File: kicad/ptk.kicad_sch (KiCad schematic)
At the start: 25 parts, among them J0 nice!view, U0 ProMicro-kbd

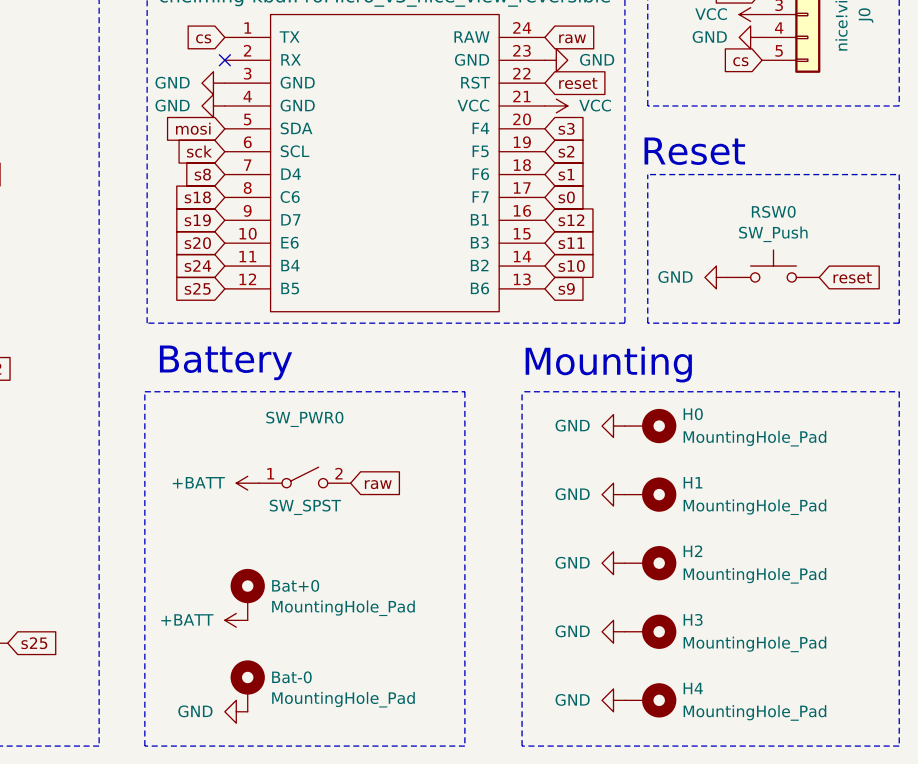
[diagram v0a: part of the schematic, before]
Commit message: add'l routing
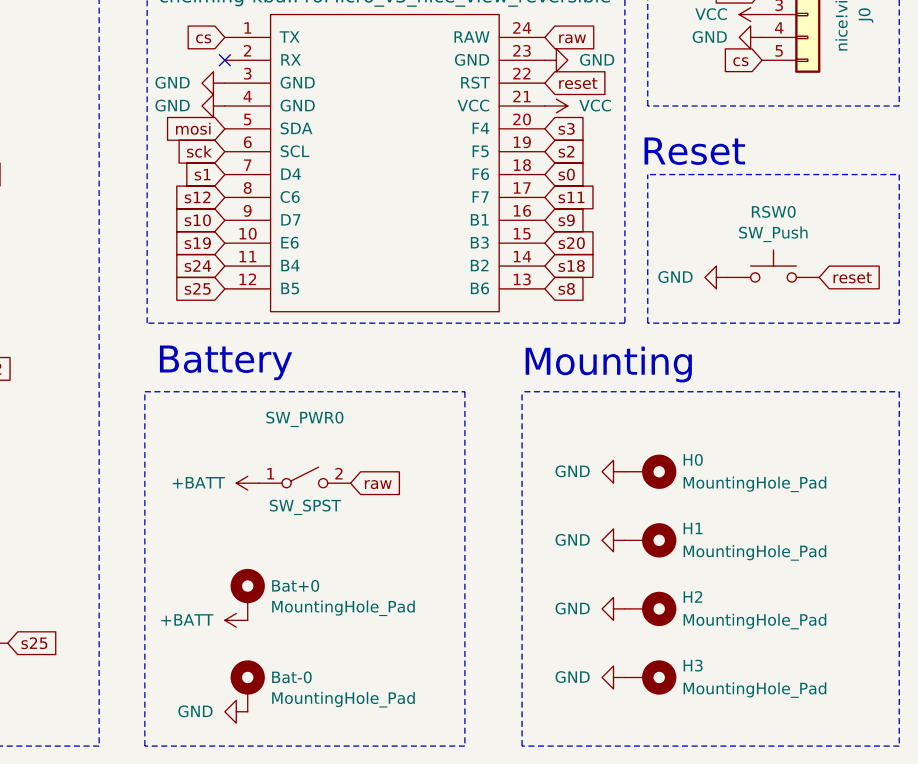
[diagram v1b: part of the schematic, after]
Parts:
- removed H4: MountingHole_Pad, MountingHole:MountingHole_2.2mm_M2_Pad_Via, symbol Mechanical:MountingHole_Pad
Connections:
- net s0: now also U0.18 (F6); no longer U0.17 (F7)
- net s1: now also U0.7 (D4); no longer U0.18 (F6)
- net s10: now also U0.9 (D7); no longer U0.14 (B2)
- net s11: now also U0.17 (F7); no longer U0.15 (B3)
- net s12: now also U0.8 (C6); no longer U0.16 (B1)
- net s18: now also U0.14 (B2); no longer U0.8 (C6)
- net s19: now also U0.10 (E6); no longer U0.9 (D7)
- net s20: now also U0.15 (B3); no longer U0.10 (E6)
- net s8: now also U0.13 (B6); no longer U0.7 (D4)
- net s9: now also U0.16 (B1); no longer U0.13 (B6)
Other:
- moved on the sheet: H0, H1, H2, H3

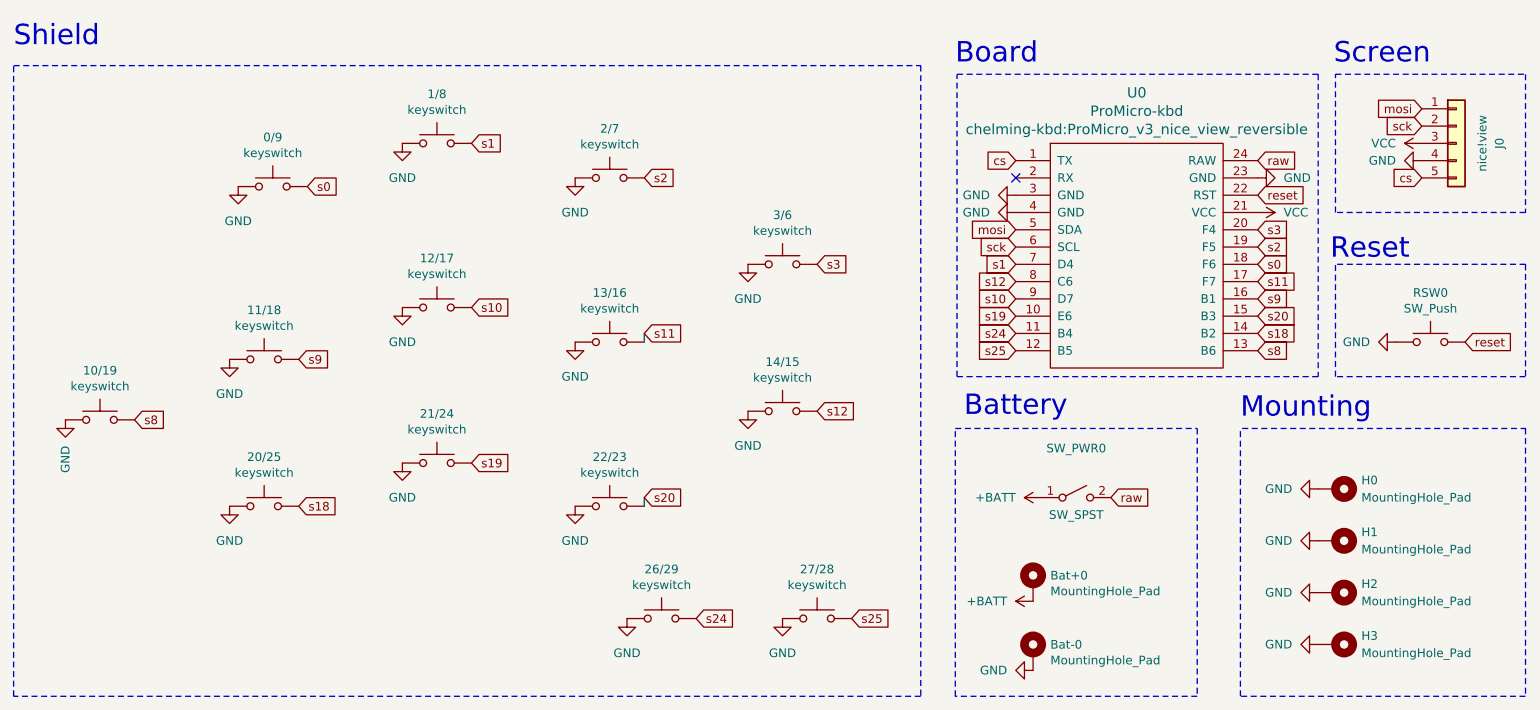
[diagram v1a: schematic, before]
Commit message: added boxes around the keys on the schematic because I'm weird like that
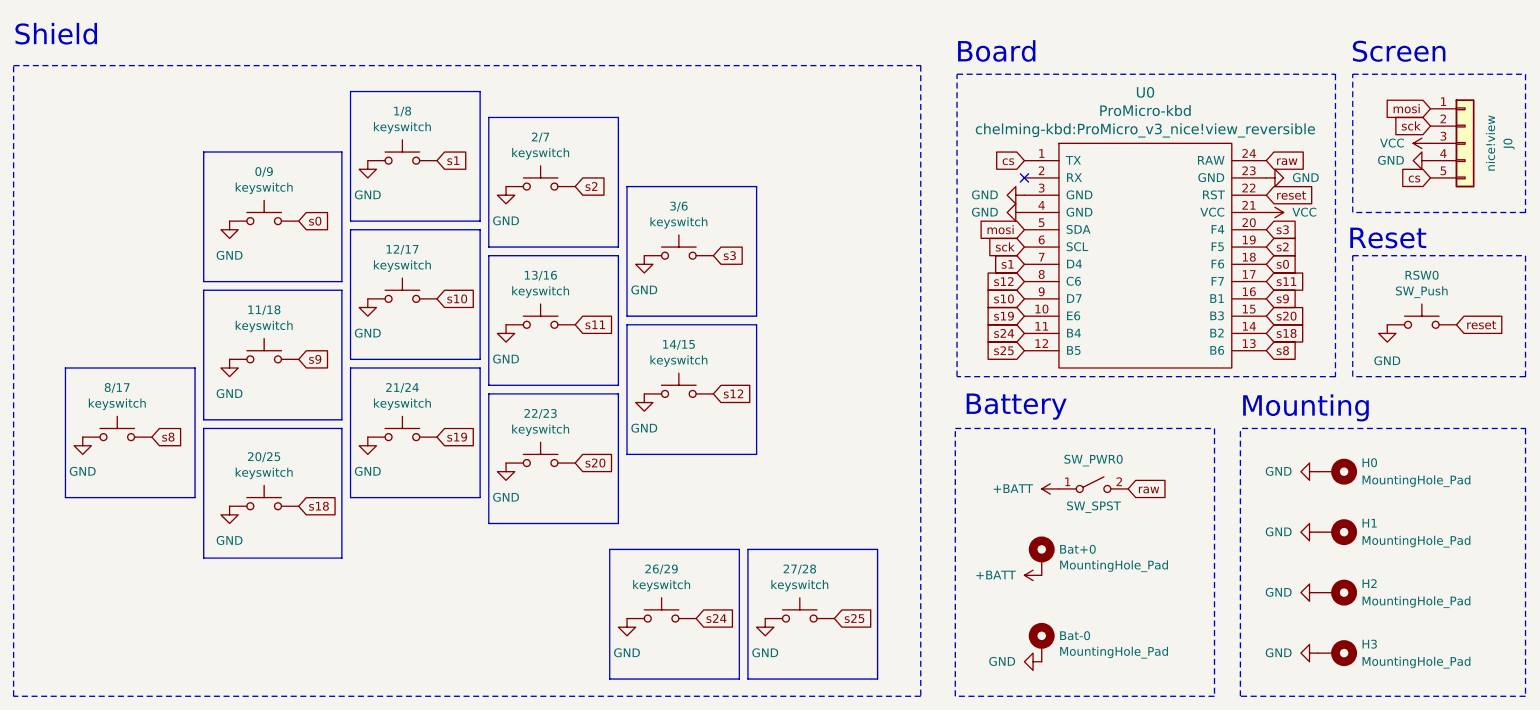
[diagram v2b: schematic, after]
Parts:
- removed 10/19: keyswitch, chelming-kbd:choc_v1_hotswap_reversible, symbol Switch:SW_Push
- added 8/17: keyswitch, chelming-kbd:choc_v1_hotswap_reversible, symbol Switch:SW_Push
- U0: footprint chelming-kbd:ProMicro_v3_nice_view_reversible -> chelming-kbd:ProMicro_v3_nice!view_reversible
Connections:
- net GND: now also 8/17.1
- net s8: now also 8/17.2
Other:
- moved on the sheet: 0/9, 1/8, 12/17, 13/16, 14/15, 2/7, 21/24, 22/23, 27/28, 3/6, Bat+0, Bat-0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
